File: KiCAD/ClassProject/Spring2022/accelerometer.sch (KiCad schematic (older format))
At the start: 14 parts, among them U12 LIS2DE12TR

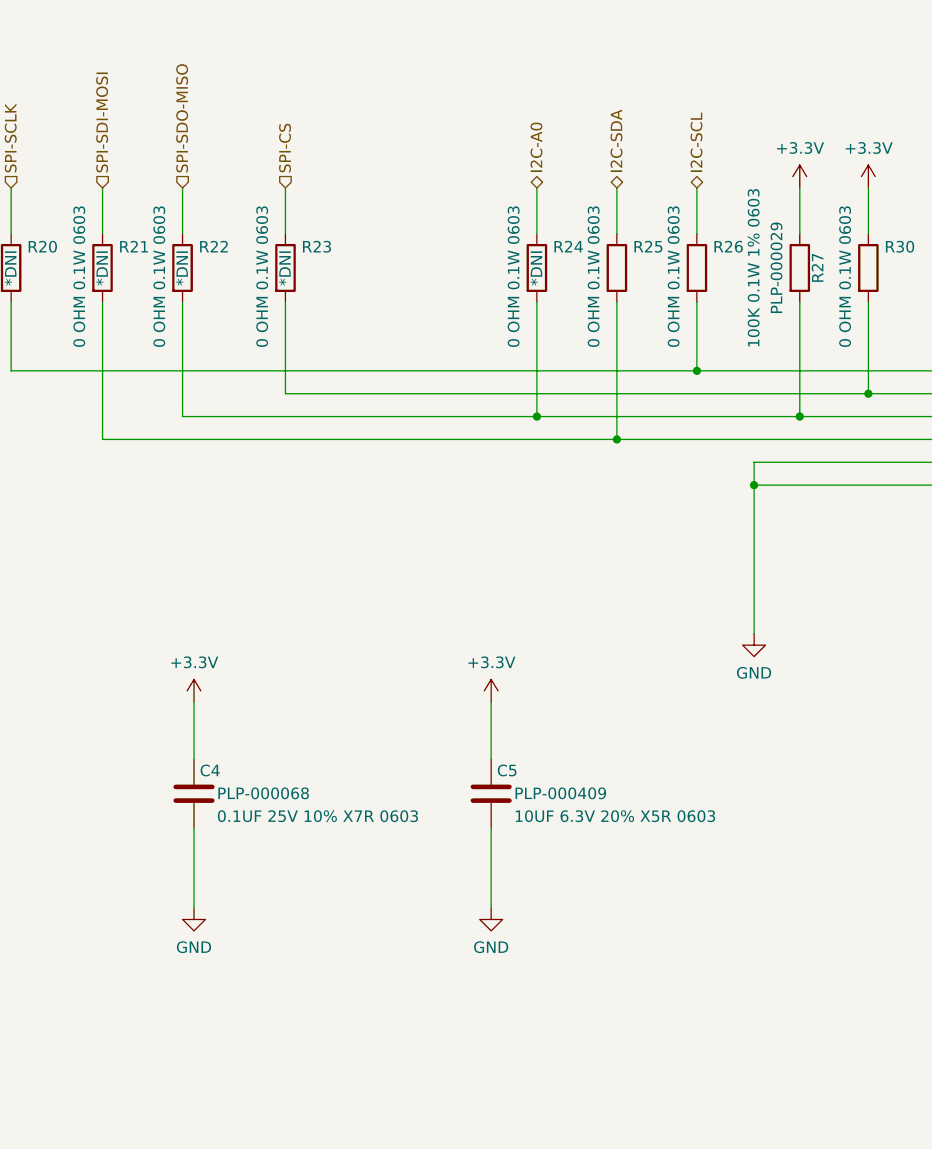
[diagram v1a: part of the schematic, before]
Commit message: PCB Layout Complete.
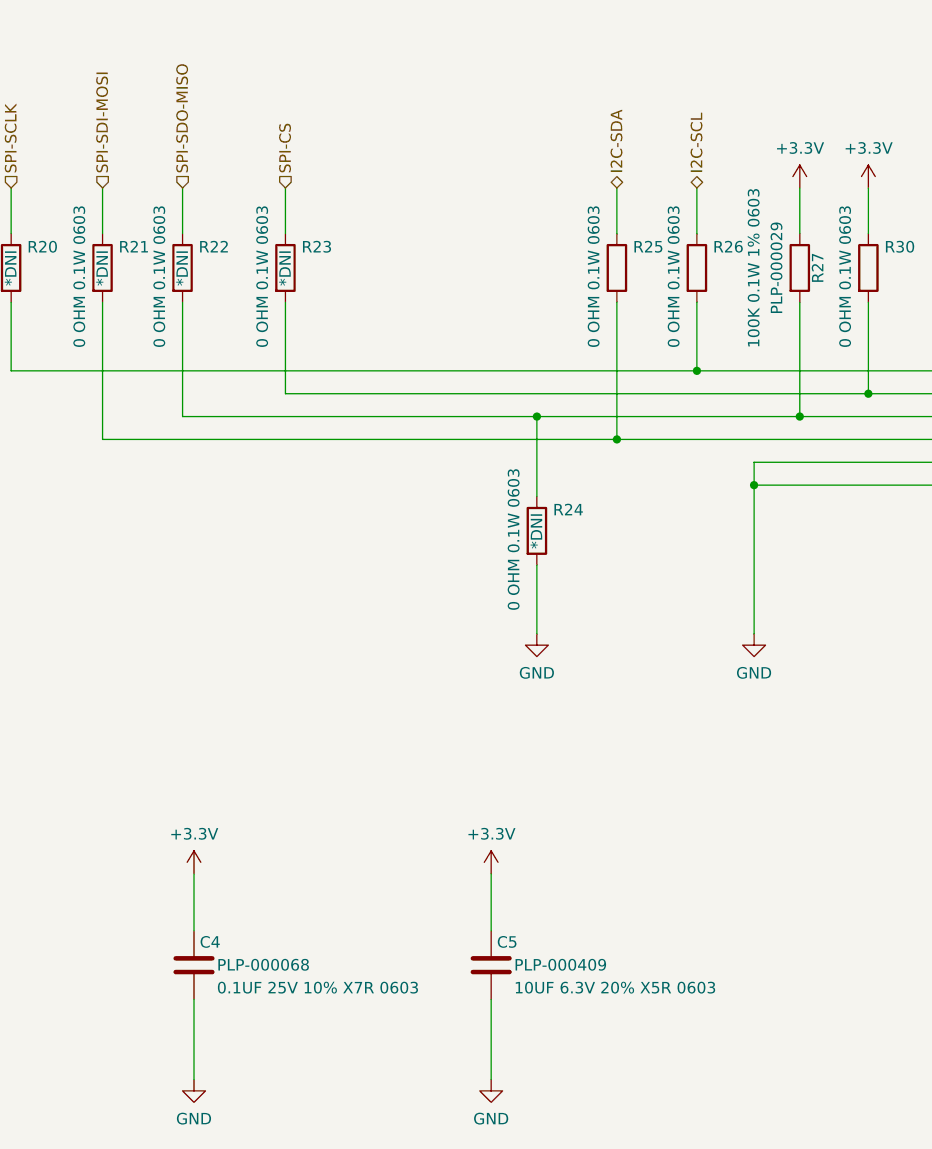
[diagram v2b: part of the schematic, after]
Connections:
- net I2C-A0 is gone; now on an unnamed net: R24.1
- net GND: now also R24.2
- net at R22.2, R27.2, U12.3 (SDO/SA0): no longer R24.2
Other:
- moved on the sheet: C4, C5, R24
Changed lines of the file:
@@
 Text HLabel 1600 2500 1    50   Input ~ 0
 SPI-SDI-MOSI
-Text HLabel 3500 2500 1    50   BiDi ~ 0
-I2C-A0
 Wire Wire Line
 	5400 3300 4200 3300
@@
 Wire Wire Line
 	3850 3600 3850 3000
-Wire Wire Line
-	3500 3500 3500 3000
 Wire Wire Line
 	1600 2500 1600 2700
@@
 L 1_pontech:PLP-000068 C4
 U 1 1 6264FAC2
-P 2000 5150
-F 0 "C4" H 2025 5250 50  0000 L CNN
-F 1 "PLP-000068" H 2100 5150 50  0000 L CNN
-F 2 "a_pontech:CAP-NON-POLAR-0603" H 2100 4700 50  0001 L CNN
-F 3 "~" H 2000 5150 50  0001 C CNN
-F 4 "0.1UF 25V 10% X7R 0603" H 2100 5050 50  0000 L CNN "Info"
-	1    2000 5150
+P 2000 5900
+F 0 "C4" H 2025 6000 50  0000 L CNN
+F 1 "PLP-000068" H 2100 5900 50  0000 L CNN
+F 2 "a_pontech:CAP-NON-POLAR-0603" H 2100 5450 50  0001 L CNN
+F 3 "~" H 2000 5900 50  0001 C CNN
+F 4 "0.1UF 25V 10% X7R 0603" H 2100 5800 50  0000 L CNN "Info"
+	1    2000 5900
 	1    0    0    -1
 $EndComp
@@
 L 1_pontech:PLP-000409 C5
 U 1 1 6264FF78
-P 3300 5150
-F 0 "C5" H 3325 5250 50  0000 L CNN
-F 1 "PLP-000409" H 3400 5150 50  0000 L CNN
-F 2 "a_pontech:CAP-NON-POLAR-0603" H 3400 4700 50  0001 L CNN
-F 3 "~" H 3300 5150 50  0001 C CNN
-F 4 "10UF 6.3V 20% X5R 0603" H 3400 5050 50  0000 L CNN "Info"
-	1    3300 5150
-	1    0    0    -1
-$EndComp
-Wire Wire Line
-	3300 5000 3300 4750
-Wire Wire Line
-	2000 5000 2000 4750
-Wire Wire Line
-	2000 5300 2000 5650
+P 3300 5900
+F 0 "C5" H 3325 6000 50  0000 L CNN
+F 1 "PLP-000409" H 3400 5900 50  0000 L CNN
+F 2 "a_pontech:CAP-NON-POLAR-0603" H 3400 5450 50  0001 L CNN
+F 3 "~" H 3300 5900 50  0001 C CNN
+F 4 "10UF 6.3V 20% X5R 0603" H 3400 5800 50  0000 L CNN "Info"
+	1    3300 5900
+	1    0    0    -1
+$EndComp
+Wire Wire Line
+	3300 5750 3300 5500
+Wire Wire Line
+	2000 5750 2000 5500
+Wire Wire Line
+	2000 6050 2000 6400
 $Comp
 L 74_Jacob:+3.3V #PWR0127
 U 1 1 626475ED
-P 2000 4750
-F 0 "#PWR0127" H 2000 4600 50  0001 C CNN
-F 1 "+3.3V" H 2000 4923 50  0000 C CNN
-F 2 "" H 2000 4750 50  0001 C CNN
-F 3 "" H 2000 4750 50  0001 C CNN
-	1    2000 4750
+P 2000 5500
+F 0 "#PWR0127" H 2000 5350 50  0001 C CNN
+F 1 "+3.3V" H 2000 5673 50  0000 C CNN
+F 2 "" H 2000 5500 50  0001 C CNN
+F 3 "" H 2000 5500 50  0001 C CNN
+	1    2000 5500
 	1    0    0    -1
 $EndComp
@@
 L 74_Jacob:+3.3V #PWR0128
 U 1 1 626484B4
-P 3300 4750
-F 0 "#PWR0128" H 3300 4600 50  0001 C CNN
-F 1 "+3.3V" H 3300 4923 50  0000 C CNN
-F 2 "" H 3300 4750 50  0001 C CNN
-F 3 "" H 3300 4750 50  0001 C CNN
-	1    3300 4750
+P 3300 5500
+F 0 "#PWR0128" H 3300 5350 50  0001 C CNN
+F 1 "+3.3V" H 3300 5673 50  0000 C CNN
+F 2 "" H 3300 5500 50  0001 C CNN
+F 3 "" H 3300 5500 50  0001 C CNN
+	1    3300 5500
 	1    0    0    -1
 $EndComp
@@
 L 74_Jacob:GND #PWR0131
 U 1 1 626496EF
-P 2000 5650
-F 0 "#PWR0131" H 2000 5400 50  0001 C CNN
-F 1 "GND" H 2000 5477 50  0000 C CNN
-F 2 "" H 2000 5650 50  0001 C CNN
-F 3 "" H 2000 5650 50  0001 C CNN
-	1    2000 5650
-	1    0    0    -1
-$EndComp
-Wire Wire Line
-	3300 5300 3300 5650
+P 2000 6400
+F 0 "#PWR0131" H 2000 6150 50  0001 C CNN
+F 1 "GND" H 2000 6227 50  0000 C CNN
+F 2 "" H 2000 6400 50  0001 C CNN
+F 3 "" H 2000 6400 50  0001 C CNN
+	1    2000 6400
+	1    0    0    -1
+$EndComp
+Wire Wire Line
+	3300 6050 3300 6400
 $Comp
 L 74_Jacob:GND #PWR0132
 U 1 1 6264A815
-P 3300 5650
-F 0 "#PWR0132" H 3300 5400 50  0001 C CNN
-F 1 "GND" H 3300 5477 50  0000 C CNN
-F 2 "" H 3300 5650 50  0001 C CNN
-F 3 "" H 3300 5650 50  0001 C CNN
-	1    3300 5650
+P 3300 6400
+F 0 "#PWR0132" H 3300 6150 50  0001 C CNN
+F 1 "GND" H 3300 6227 50  0000 C CNN
+F 2 "" H 3300 6400 50  0001 C CNN
+F 3 "" H 3300 6400 50  0001 C CNN
+	1    3300 6400
 	1    0    0    -1
 $EndComp
@@
 L 1_pontech:PLP-000091 R24
 U 1 1 62663FDF
-P 3500 2850
-F 0 "R24" H 3570 2941 50  0000 L CNN
-F 1 "PLP-000091" H 3570 2850 50  0001 L CNN
-F 2 "a_pontech:R_0603_1608Metric" V 3430 2850 50  0001 C CNN
-F 3 "~" H 3500 2850 50  0001 C CNN
-F 4 "0 OHM 0.1W 0603" V 3400 2500 50  0000 L CNN "Info"
-F 5 "*DNI" V 3500 2850 50  0000 C CNN "DNI"
-	1    3500 2850
-	1    0    0    -1
-$EndComp
-Wire Wire Line
-	3500 2700 3500 2500
+P 3500 4000
+F 0 "R24" H 3570 4091 50  0000 L CNN
+F 1 "PLP-000091" H 3570 4000 50  0001 L CNN
+F 2 "a_pontech:R_0603_1608Metric" V 3430 4000 50  0001 C CNN
+F 3 "~" H 3500 4000 50  0001 C CNN
+F 4 "0 OHM 0.1W 0603" V 3400 3650 50  0000 L CNN "Info"
+F 5 "*DNI" V 3500 4000 50  0000 C CNN "DNI"
+	1    3500 4000
+	1    0    0    -1
+$EndComp
 $Comp
 L 1_pontech:PLP-000091 R25
@@
 	1    0    0    -1
 $EndComp
+$Comp
+L 74_Jacob:GND #PWR?
+U 1 1 6277FCB9
+P 3500 4450
+F 0 "#PWR?" H 3500 4200 50  0001 C CNN
+F 1 "GND" H 3500 4277 50  0000 C CNN
+F 2 "" H 3500 4450 50  0001 C CNN
+F 3 "" H 3500 4450 50  0001 C CNN
+	1    3500 4450
+	1    0    0    -1
+$EndComp
+Wire Wire Line
+	3500 4150 3500 4450
+Wire Wire Line
+	3500 3850 3500 3500
 $EndSCHEMATC
